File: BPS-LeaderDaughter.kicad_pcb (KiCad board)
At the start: 2 copper layers, 50 x 131 mm, 100 parts, among them IC1 ADT7470ARQZ-REEL7, J1 DaughterConnector, J10 Conn_01x04, J11 Conn_01x04, J12 Conn_01x04, J2 DaughterConnector, J3 ErrorLightConn, J4 Conn_01x04, J5 Conn_01x04, J6 Conn_01x04, J7 Conn_01x04, J8 Conn_01x03, J9 Conn_01x04, Q1 BUK9M23-80E, Q2 BUK9M23-80E, Q3 BUK9M23-80E, Q4 BUK9M23-80E, Q5 BUK9M23-80E, Q6 BUK9M23-80E, Q7 BUK9M23-80E, Q8 BUK9M23-80E, U1 EL3H7, U2 EL3H7

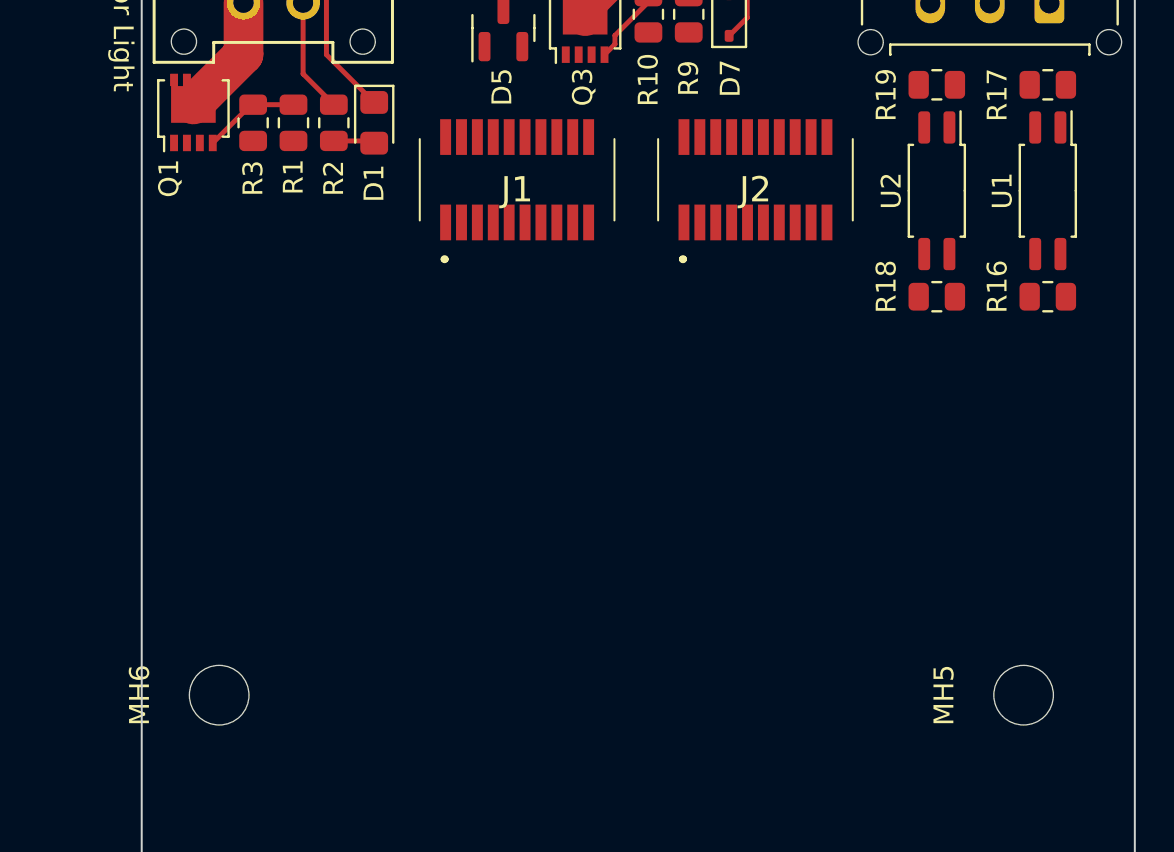
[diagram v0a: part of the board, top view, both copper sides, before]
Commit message: center som board
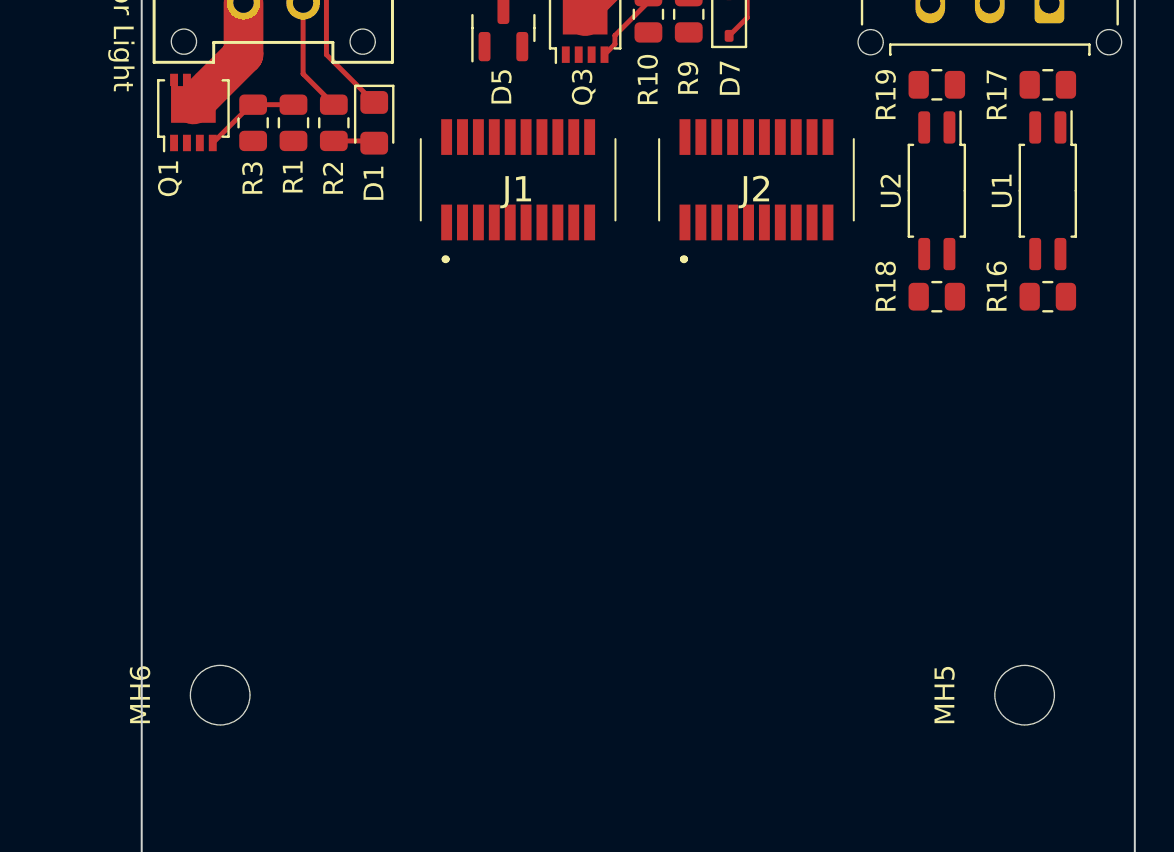
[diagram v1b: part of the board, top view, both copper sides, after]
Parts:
- moved J1 0.05 mm to (110.0, 117.4)
- moved J2 0.05 mm to (122.0, 117.4)
- moved MH5 0.05 mm to (135.5, 143.3)
- moved MH6 0.05 mm to (95.0, 143.3)
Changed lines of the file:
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@@
   )
   (footprint "MountingHole:MountingHole_3mm" (layer "F.Cu")
-    (at 94.9 143.35 90)
+    (at 94.951 143.35 90)
     (descr "Mounting Hole 3mm, no annular")
     (tags "mounting hole 3mm no annular")
@@
   )
   (footprint "UTSVT_Connectors:533072071" (layer "F.Cu")
-    (at 121.9 117.4 180)
+    (at 121.951 117.4 180)
     (descr "53307-2071-2")
     (tags "Connector")
@@
   )
   (footprint "MountingHole:MountingHole_3mm" (layer "F.Cu")
-    (at 135.4 143.35 90)
+    (at 135.451 143.35 90)
     (descr "Mounting Hole 3mm, no annular")
     (tags "mounting hole 3mm no annular")
@@
   )
   (footprint "UTSVT_Connectors:533072071" (layer "F.Cu")
-    (at 109.9 117.4 180)
+    (at 109.951 117.4 180)
     (descr "53307-2071-2")
     (tags "Connector")
@@
   (gr_line (start 267.57 22.68) (end 261.57 22.68)
     (stroke (width 0.15) (type default)) (layer "F.SilkS"))
-  (gr_line (start 132.9 119.4) (end 132.9 135.4)
+  (gr_line (start 132.951 119.4) (end 132.951 135.4)
     (stroke (width 0.15) (type default)) (layer "Dwgs.User"))
-  (gr_line (start 132.9 135.4) (end 140.9 135.4)
+  (gr_line (start 132.951 135.4) (end 140.951 135.4)
     (stroke (width 0.15) (type default)) (layer "Dwgs.User"))
-  (gr_line (start 140.9 119.4) (end 132.9 119.4)
+  (gr_line (start 140.951 119.4) (end 132.951 119.4)
     (stroke (width 0.15) (type default)) (layer "Dwgs.User"))
   (gr_rect (start 91 50.05) (end 141 181.05)
     (stroke (width 0.1) (type default)) (fill none) (layer "Edge.Cuts"))
-  (gr_arc (start 94.9 173.35) (mid 92.071573 172.178427) (end 90.9 169.35)
+  (gr_arc (start 94.951 173.35) (mid 92.122573 172.178427) (end 90.951 169.35)
     (stroke (width 0.1) (type default)) (layer "User.1"))
-  (gr_line (start 127.4 113.35) (end 136.9 113.35)
+  (gr_line (start 127.451 113.35) (end 136.951 113.35)
     (stroke (width 0.1) (type default)) (layer "User.1"))
-  (gr_line (start 105.4 112.35) (end 126.4 112.35)
+  (gr_line (start 105.451 112.35) (end 126.451 112.35)
     (stroke (width 0.1) (type default)) (layer "User.1"))
-  (gr_line (start 140.9 169.35) (end 140.9 117.35)
+  (gr_line (start 140.951 169.35) (end 140.951 117.35)
     (stroke (width 0.1) (type default)) (layer "User.1"))
-  (gr_line (start 104.4 113.35) (end 105.4 112.35)
+  (gr_line (start 104.451 113.35) (end 105.451 112.35)
     (stroke (width 0.1) (type default)) (layer "User.1"))
-  (gr_arc (start 140.9 169.35) (mid 139.728427 172.178427) (end 136.9 173.35)
+  (gr_arc (start 140.951 169.35) (mid 139.779427 172.178427) (end 136.951 173.35)
     (stroke (width 0.1) (type default)) (layer "User.1"))
-  (gr_line (start 126.4 112.35) (end 127.4 113.35)
+  (gr_line (start 126.451 112.35) (end 127.451 113.35)
     (stroke (width 0.1) (type default)) (layer "User.1"))
-  (gr_line (start 94.9 173.35) (end 136.9 173.35)
+  (gr_line (start 94.951 173.35) (end 136.951 173.35)
     (stroke (width 0.1) (type default)) (layer "User.1"))
-  (gr_line (start 90.9 169.35) (end 90.9 117.35)
+  (gr_line (start 90.951 169.35) (end 90.951 117.35)
     (stroke (width 0.1) (type default)) (layer "User.1"))
-  (gr_arc (start 90.9 117.35) (mid 92.071573 114.521573) (end 94.9 113.35)
+  (gr_arc (start 90.951 117.35) (mid 92.122573 114.521573) (end 94.951 113.35)
     (stroke (width 0.1) (type default)) (layer "User.1"))
-  (gr_arc (start 136.9 113.35) (mid 139.728427 114.521573) (end 140.9 117.35)
+  (gr_arc (start 136.951 113.35) (mid 139.779427 114.521573) (end 140.951 117.35)
     (stroke (width 0.1) (type default)) (layer "User.1"))
-  (gr_line (start 94.9 113.35) (end 104.4 113.35)
+  (gr_line (start 94.951 113.35) (end 104.451 113.35)
     (stroke (width 0.1) (type default)) (layer "User.1"))
   (gr_text "FAN 1\n" (at 110.744 67.564 90) (layer "F.SilkS")
@@
     (effects (font (size 1 1) (thickness 0.15)) (justify left bottom))
   )
-  (gr_text "USB" (at 137.9 129.4 90) (layer "Dwgs.User")
+  (gr_text "USB" (at 137.951 129.4 90) (layer "Dwgs.User")
     (effects (font (size 1 1) (thickness 0.15)) (justify left bottom))
   )
   (dimension (type aligned) (layer "Dwgs.User")
-    (pts (xy 135.4 143.35) (xy 140.9 143.35))
+    (pts (xy 135.451 143.35) (xy 140.951 143.35))
     (height 7)
-    (gr_text "5.5000 mm" (at 138.15 149.2) (layer "Dwgs.User")
+    (gr_text "5.5000 mm" (at 138.201 149.2) (layer "Dwgs.User")
       (effects (font (size 1 1) (thickness 0.15)))
     )
@@
   )
   (dimension (type aligned) (layer "Dwgs.User")
-    (pts (xy 94.9 143.35) (xy 90.9 143.35))
+    (pts (xy 94.951 143.35) (xy 90.951 143.35))
     (height -7)
-    (gr_text "4.0000 mm" (at 92.9 149.2) (layer "Dwgs.User")
+    (gr_text "4.0000 mm" (at 92.951 149.2) (layer "Dwgs.User")
       (effects (font (size 1 1) (thickness 0.15)))
     )
@@
   )
   (dimension (type aligned) (layer "Dwgs.User")
-    (pts (xy 135.4 143.35) (xy 94.9 143.35))
+    (pts (xy 135.451 143.35) (xy 94.951 143.35))
     (height 0)
-    (gr_text "40.5000 mm" (at 115.15 142.2) (layer "Dwgs.User")
+    (gr_text "40.5000 mm" (at 115.201 142.2) (layer "Dwgs.User")
       (effects (font (size 1 1) (thickness 0.15)))
     )
